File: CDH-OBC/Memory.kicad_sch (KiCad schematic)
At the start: 47 parts, among them J1 Conn_01x04, SW1 SW_Push, SW2 SW_Push, U2 MR25H256AMDF, U3 TPS3850H50DRCR, U4 W25N02KVZEIR, U5 PCA2129T/Q900/2_51, U6 SN65HVD230, U7 S25FL128LAGMFM010

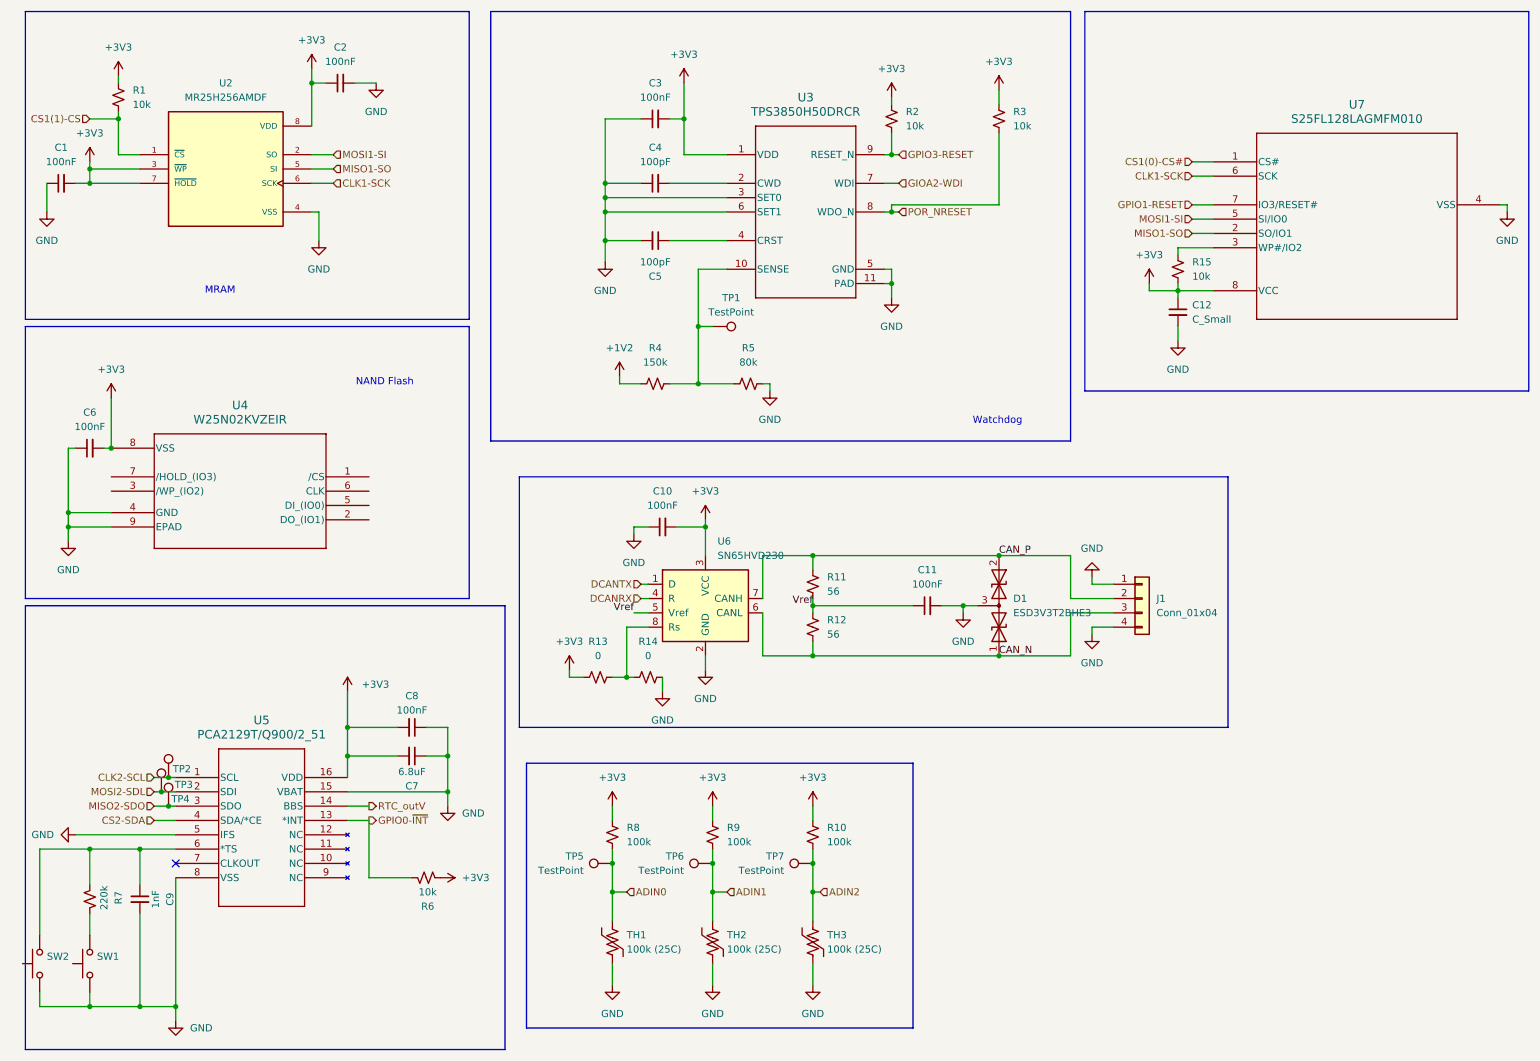
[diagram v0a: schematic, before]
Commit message: finished bulk of the schematic
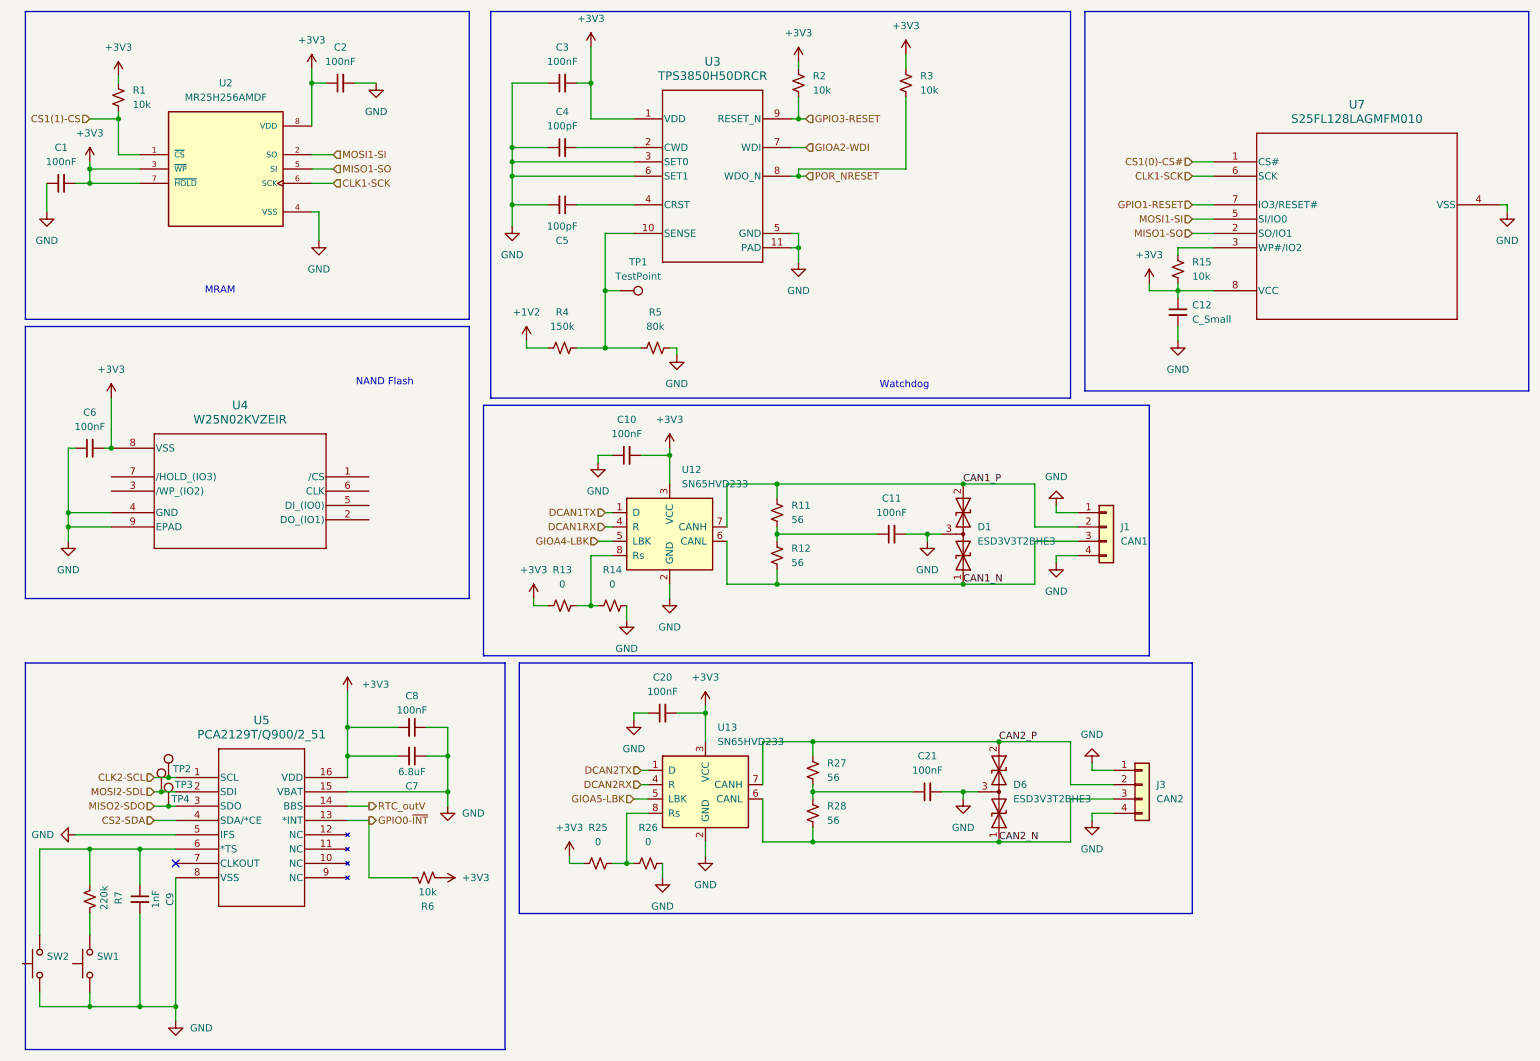
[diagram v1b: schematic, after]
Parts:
- removed R10, R8, R9: 100k, symbol Device:R_Small_US
- removed TH1, TH2, TH3: 100k (25C), symbol Device:Thermistor_US
- removed TP5, TP6, TP7: TestPoint, symbol Connector:TestPoint
- removed U6: SN65HVD230, Package_SO:SOIC-8_3.9x4.9mm_P1.27mm, symbol Interface_CAN_LIN:SN65HVD230
- added C20, C21: 100nF, symbol Device:C_Small
- added D6: ESD3V3T2BHE3, symbol Device:D_TVS_Dual_AAC
- added J3: CAN2, symbol Connector_Generic:Conn_01x04
- added R25, R26: 0, symbol Device:R_Small_US
- added R27, R28: 56, symbol Device:R_Small_US
- added U12, U13: SN65HVD233, Package_SO:SOIC-8_3.9x4.9mm_P1.27mm, symbol Interface_CAN_LIN:SN65HVD233
- J1: value Conn_01x04 -> CAN1
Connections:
- net +3V3: now also C20.2, R25.1, U12.3 (VCC), U13.3 (VCC)
- net GND: now also C20.1, C21.2, D6.3 (common), J3.1 (Pin_1), J3.4 (Pin_4), R26.2, U12.2 (GND), U13.2 (GND)
- net at R13.2, R14.1: now also U12.8 (Rs)
- net CAN_N renamed CAN1_N
- net CAN1_N: now also U12.6 (CANL)
- net CAN_P renamed CAN1_P
- net CAN1_P: now also U12.7 (CANH)
- net Vref: no longer names the net of C11.1, R11.2, R12.1
- new net: C21.1, R27.2, R28.1
- new net: R25.2, R26.1, U13.8 (Rs)
- new net CAN2_N: D6.1 (A1), J3.3 (Pin_3), R28.2, U13.6 (CANL)
- new net CAN2_P: D6.2 (A2), J3.2 (Pin_2), R27.1, U13.7 (CANH)
- new net DCAN1RX: U12.4 (R)
- new net DCAN1TX: U12.1 (D)
- new net DCAN2RX: U13.4 (R)
- new net DCAN2TX: U13.1 (D)
- new net GIOA4-LBK: U12.5 (LBK)
- new net GIOA5-LBK: U13.5 (LBK)
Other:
- moved on the sheet: C10, C11, C3, C4, C5, D1, J1, R11, R12, R13, R14, R2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
